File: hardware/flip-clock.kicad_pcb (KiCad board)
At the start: 2 copper layers, 64 x 53.3 mm, 12 parts, among them J1 Screw_Terminal_01x02, J2 Conn_01x03_Female, U1 WeMos_D1_mini

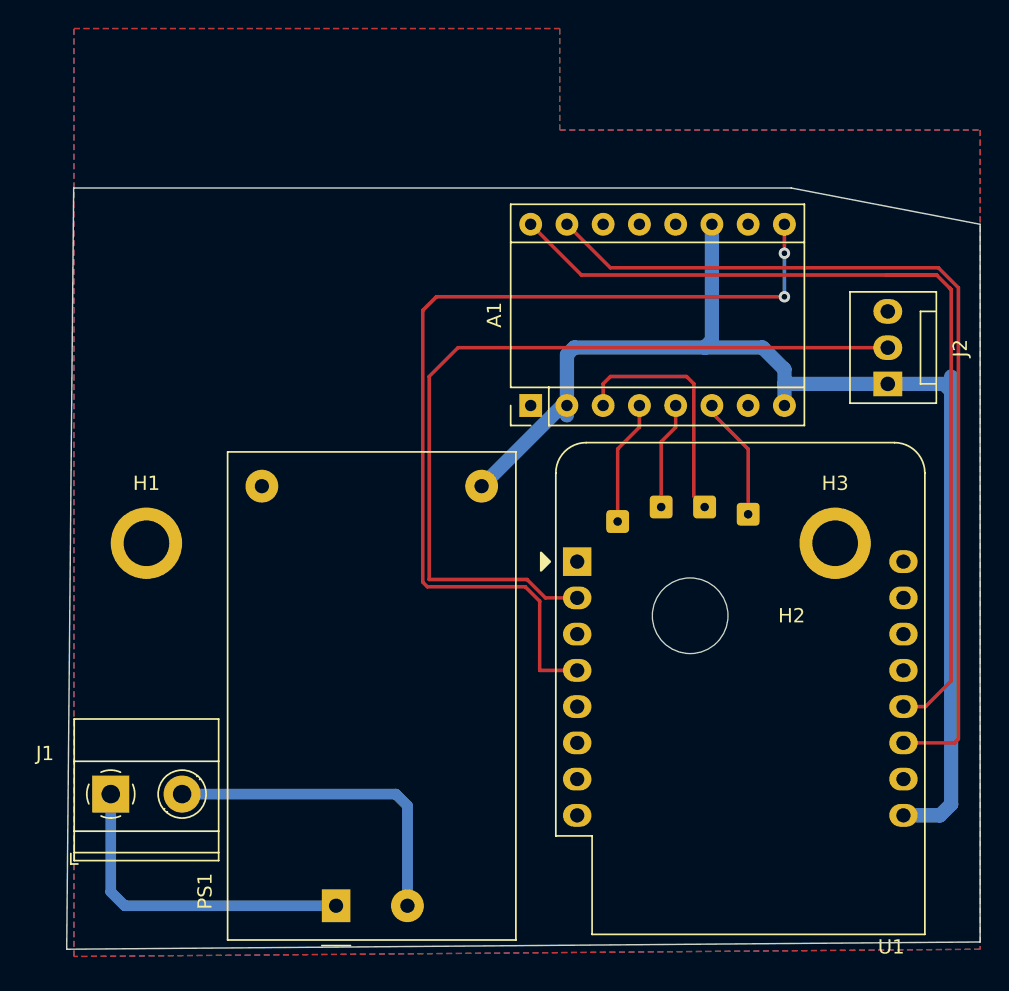
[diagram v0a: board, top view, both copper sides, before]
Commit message: Correct side
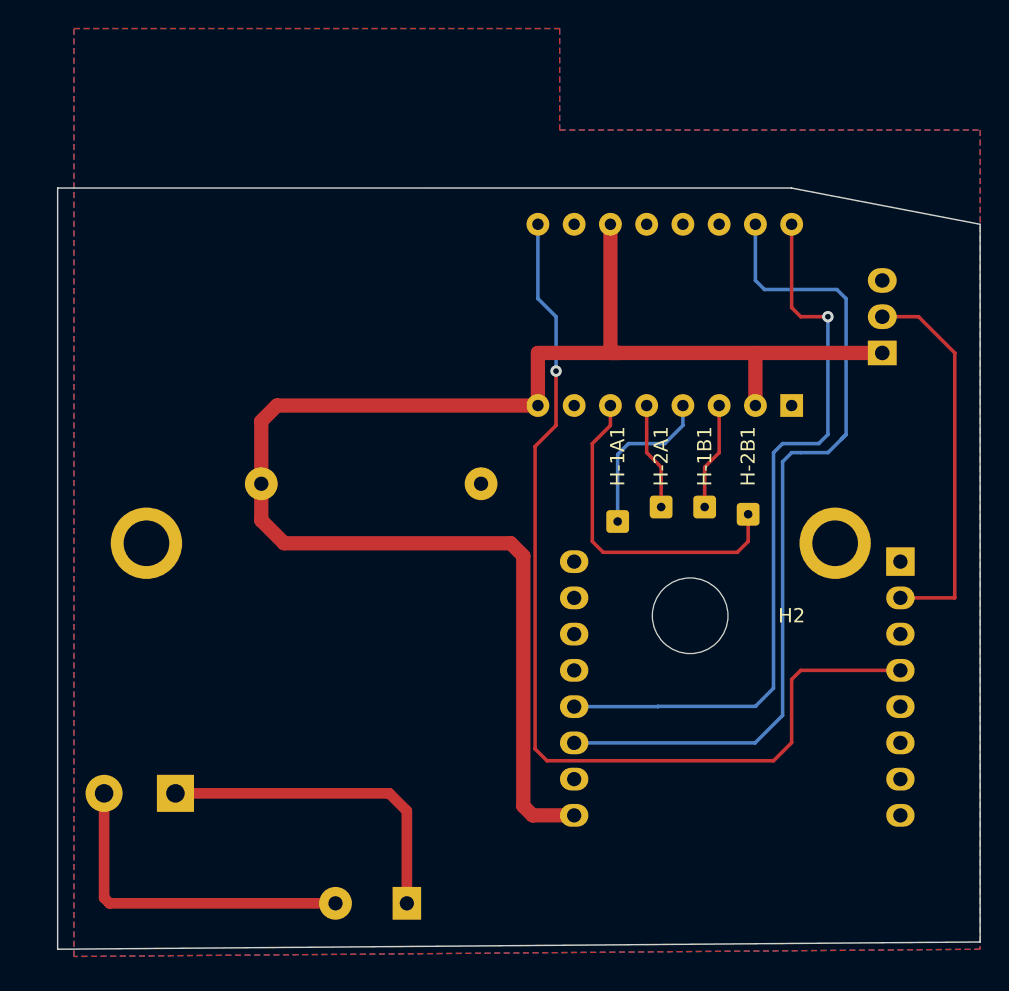
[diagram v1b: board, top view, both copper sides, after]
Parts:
- A1, H1, H3, J1, J2, PS1, U1: moved to B.Cu
- moved U1 22.6 mm to (172.7, 57.2), turned to 180 degrees
- moved A1 18.3 mm to (165.1, 46.2)
- moved PS1 4.96 mm to (138.1, 81.1)
- moved J1 4.53 mm to (121.9, 73.4), turned to 180 degrees
- moved J2 2.20 mm to (171.4, 42.5)
- turned H1 to 180 degrees
- turned H3 to 180 degrees
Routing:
- net /PD_IN: track 58.1 -> 27.1 mm
- net VCC: track 85.7 -> 108.7 mm
- net /2B: track 8.67 -> 23.5 mm
- net /DIR: track 66.6 -> 52.2 mm, vias 0 -> 1
- net /1B: track 17.2 -> 7.53 mm
- net /STEP: track 64.9 -> 59.2 mm
- net //ENABLE: track 66.1 -> 69.1 mm, vias 2 -> 1
- net /1A: track 8.76 -> 11.5 mm
- net /AC1: track 23.1 -> 23.7 mm
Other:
- board size 64 x 53.3 mm -> 64.6 x 53.3 mm
